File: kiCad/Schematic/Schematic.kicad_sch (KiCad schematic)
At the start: 8 parts, among them J1 BAT, J2 Switch, J3 MPU 6050, J4 ESP 32, J5 UltraSonic Sensor, J6 BUCK CONVERTER, M1 Stepper_Motor_bipolar, M2 Stepper_Motor_bipolar

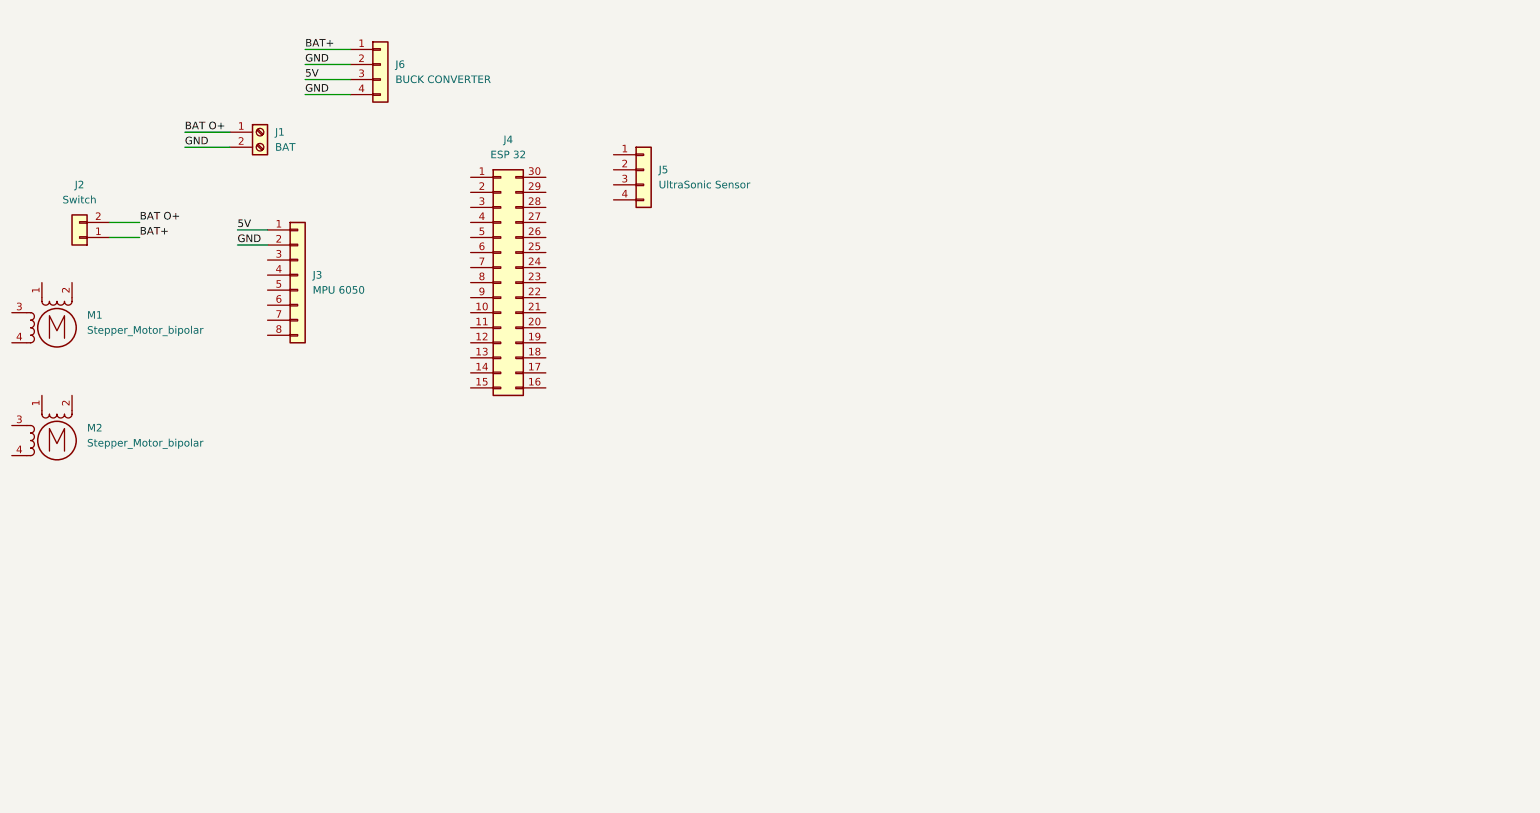
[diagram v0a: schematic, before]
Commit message: Day 3: Part one
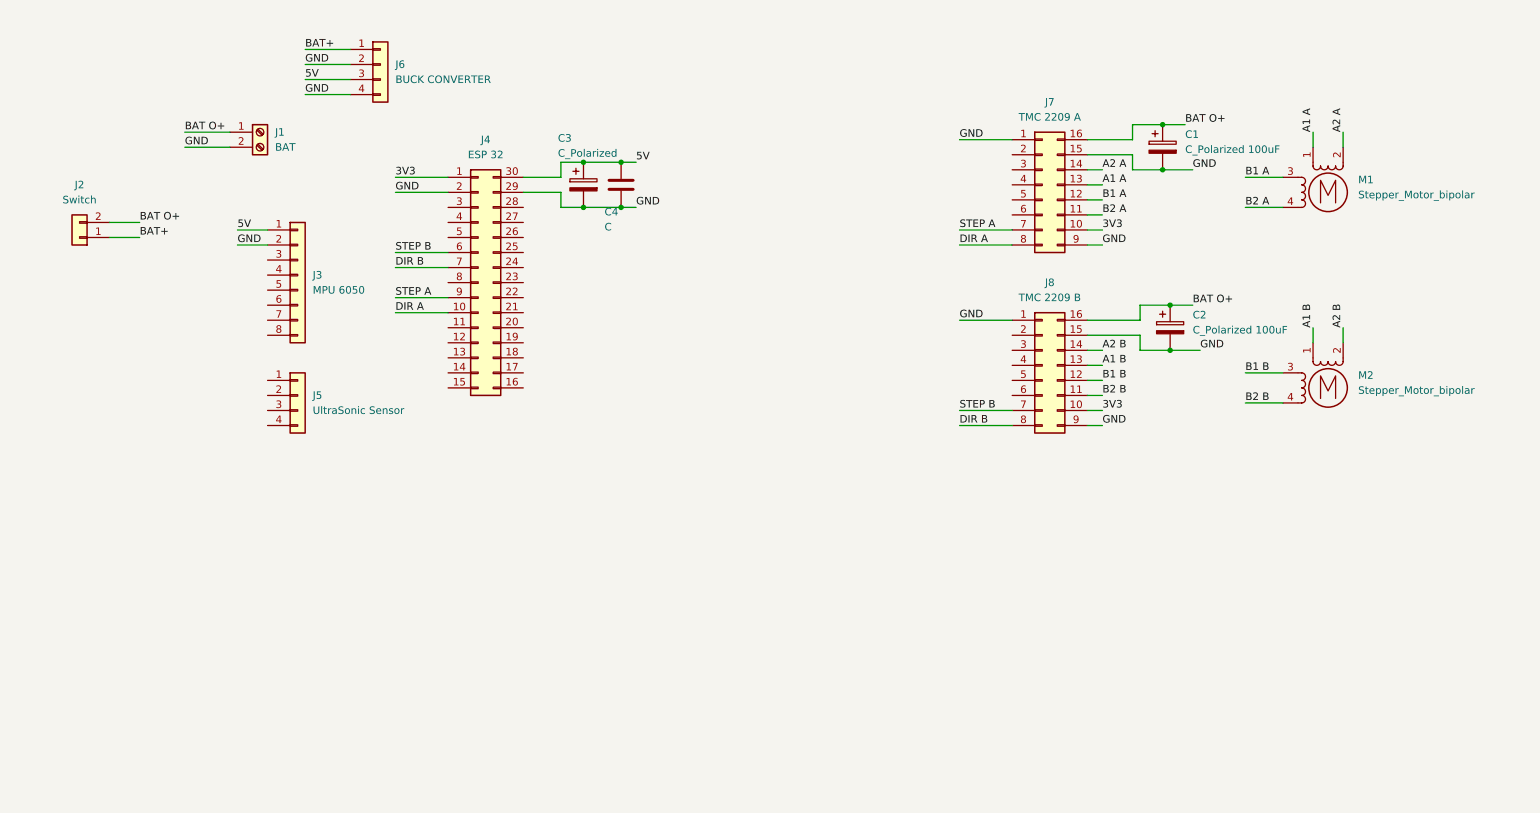
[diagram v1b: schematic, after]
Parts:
- added C1, C2: C_Polarized 100uF, symbol Device:C_Polarized
- added C3: C_Polarized, symbol Device:C_Polarized
- added C4: C, symbol Device:C
- added J7: TMC 2209 A, symbol Connector_Generic:Conn_02x08_Counter_Clockwise
- added J8: TMC 2209 B, symbol Connector_Generic:Conn_02x08_Counter_Clockwise
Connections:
- net 5V: now also J4.30 (Pin_30), C3.1, C4.1
- net BAT O+: now also C1.1, C2.1, J7.16 (Pin_16), J8.16 (Pin_16)
- net GND: now also J4.2 (Pin_2), J4.29 (Pin_29), C1.2, C2.2, C3.2, C4.2, J7.1 (Pin_1), J7.15 (Pin_15), J7.9 (Pin_9), J8.1 (Pin_1), J8.15 (Pin_15), J8.9 (Pin_9)
- net A1 B: now reaches M2.1
- net A1 B: now also J8.13 (Pin_13)
- net A2 B: now reaches M2.2 (-)
- net A2 B: now also J8.14 (Pin_14)
- net B1 B: now reaches M2.3
- net B1 B: now also J8.12 (Pin_12)
- net B2 B: now reaches M2.4
- net B2 B: now also J8.11 (Pin_11)
- net A1 A: now reaches M1.1
- net A1 A: now also J7.13 (Pin_13)
- net A2 A: now reaches M1.2 (-)
- net A2 A: now also J7.14 (Pin_14)
- net B1 A: now reaches M1.3
- net B1 A: now also J7.12 (Pin_12)
- net B2 A: now reaches M1.4
- net B2 A: now also J7.11 (Pin_11)
- net 3V3: now reaches J4.1 (Pin_1)
- net 3V3: now also J7.10 (Pin_10), J8.10 (Pin_10)
- net DIR A: now reaches J4.10 (Pin_10)
- net DIR A: now also J7.8 (Pin_8)
- net STEP B: now reaches J4.6 (Pin_6)
- net STEP B: now also J8.7 (Pin_7)
- net DIR B: now reaches J4.7 (Pin_7)
- net DIR B: now also J8.8 (Pin_8)
- net STEP A: now reaches J4.9 (Pin_9)
- net STEP A: now also J7.7 (Pin_7)
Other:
- moved on the sheet: J4, J5, M1, M2

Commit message: Day 3: Schematic done
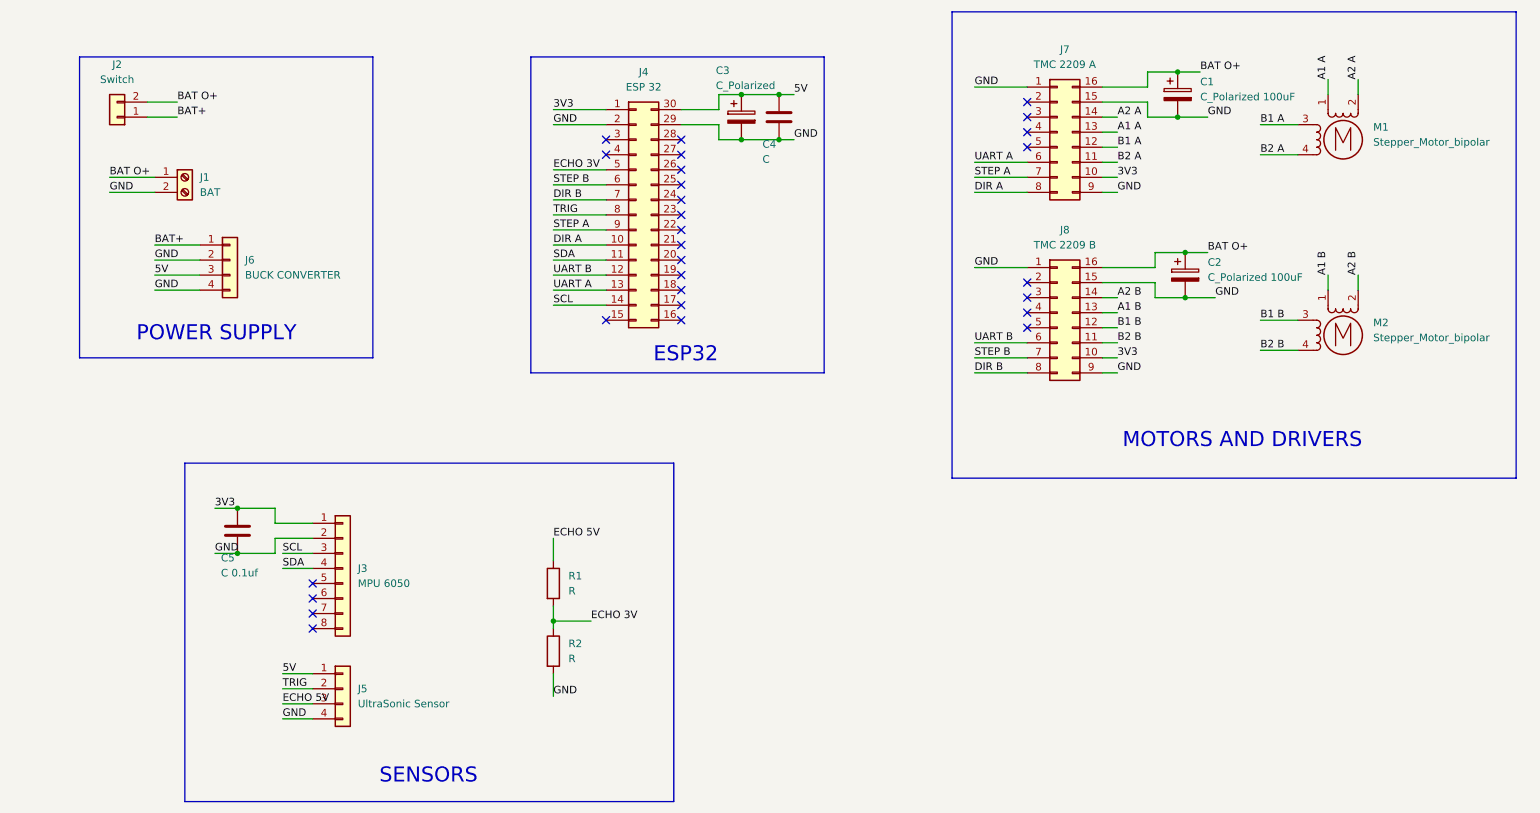
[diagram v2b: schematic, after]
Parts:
- added C5: C 0.1uf, symbol Device:C
- added R1, R2: R, symbol Device:R
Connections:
- net 3V3: now also J3.1 (Pin_1), C5.1
- net 5V: now also J5.1 (Pin_1); no longer J3.1 (Pin_1)
- net GND: now also J5.4 (Pin_4), C5.2, R2.2
- net SCL: now reaches J3.3 (Pin_3)
- net SCL: now also J4.14 (Pin_14)
- net SDA: now reaches J3.4 (Pin_4)
- net SDA: now also J4.11 (Pin_11)
- net UART A: now reaches J7.6 (Pin_6)
- net UART A: now also J4.13 (Pin_13)
- net TRIG: now reaches J5.2 (Pin_2)
- net TRIG: now also J4.8 (Pin_8)
- net ECHO 5V: now reaches J5.3 (Pin_3)
- net ECHO 5V: now also R1.1
- net UART B: now reaches J4.12 (Pin_12)
- net UART B: now also J8.6 (Pin_6)
- net ECHO 3V: now reaches J4.5 (Pin_5)
- net ECHO 3V: now also R1.2, R2.1
- no-connect marks 0 -> 28
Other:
- note added: "ESP32"
- note added: "MOTORS AND DRIVERS"
- note added: "POWER SUPPLY"
- note added: "SENSORS"
- moved on the sheet: C1, C2, C3, C4, J1, J2, J3, J4, J5, J6, J7, J8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
